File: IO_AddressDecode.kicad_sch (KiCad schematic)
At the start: 42 parts, among them J0 Cassette Data In, J13 74LS74, J14 GAME_IO_Conn, J2 Cassette Data Out, K13 MA741, Q4 MPSA13

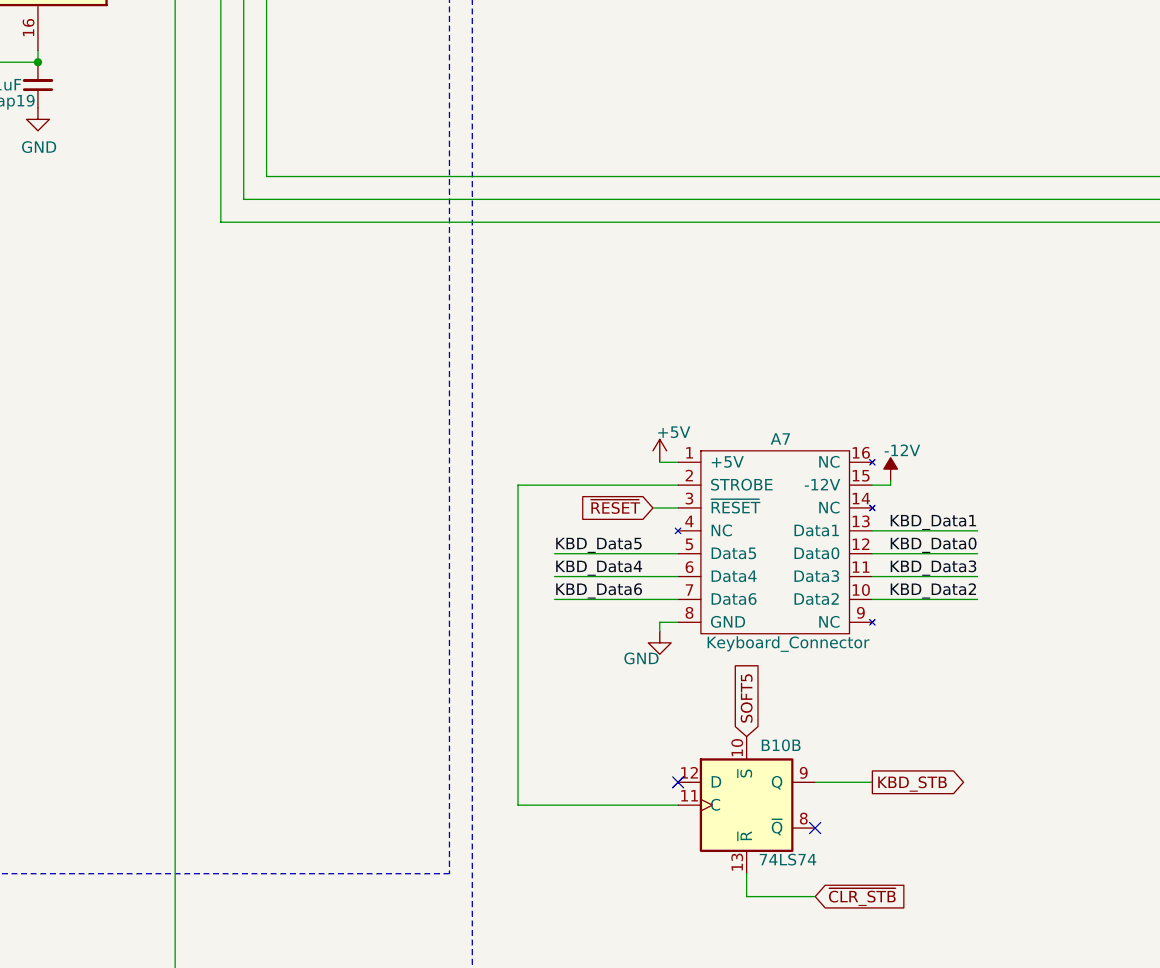
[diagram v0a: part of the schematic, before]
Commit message: finish tracing
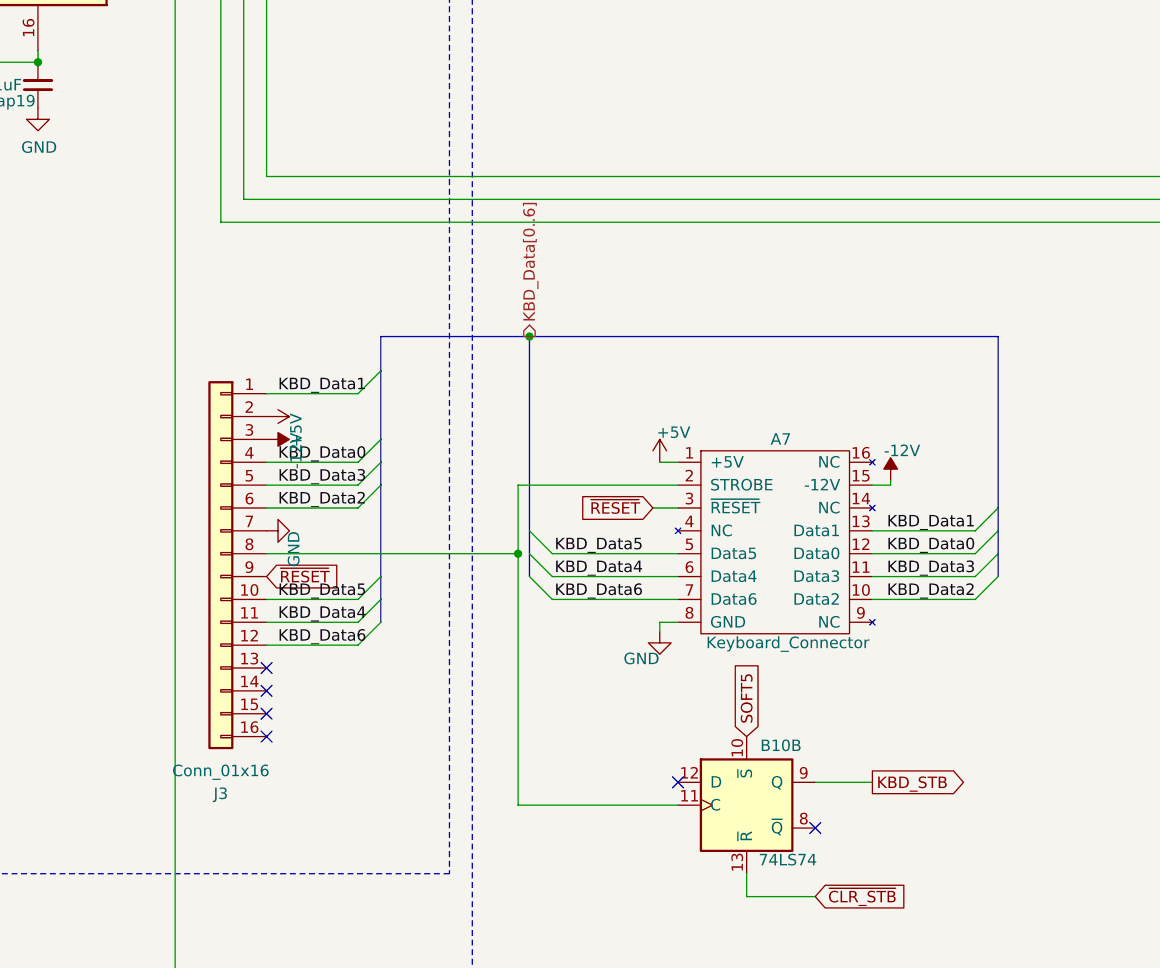
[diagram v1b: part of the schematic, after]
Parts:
- added J3: Conn_01x16, Connector_PinHeader_2.54mm:PinHeader_1x16_P2.54mm_Vertical, symbol Connector_Generic:Conn_01x16
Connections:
- net +5V: now also J3.2 (Pin_2)
- net -12V: now also J3.3 (Pin_3)
- net GND: now also J3.7 (Pin_7)
- net KBD_Data0: now also J3.4 (Pin_4)
- net KBD_Data1: now also J3.1 (Pin_1)
- net KBD_Data2: now also J3.6 (Pin_6)
- net KBD_Data3: now also J3.5 (Pin_5)
- net KBD_Data4: now also J3.11 (Pin_11)
- net KBD_Data5: now also J3.10 (Pin_10)
- net KBD_Data6: now also J3.12 (Pin_12)
- net ~{RESET}: now also J3.9 (Pin_9)
- net at A7.2 (STROBE), B10.11 (C): now also J3.8 (Pin_8)
- no-connect marks 7 -> 11

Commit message: beautify resistors
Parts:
- Cap10, Cap11, Cap12, Cap16, Cap18, Cap19, Cap5, Cap6, Cap7, Cap9: footprint Capacitor_THT:C_Disc_D5.0mm_W2.5mm_P5.00mm -> Apple-II:C_Disc_D5.0mm_W2.5mm_P5.00mm
- Cap8: footprint Capacitor_THT:C_Disc_D4.3mm_W1.9mm_P5.00mm -> Apple-II:C_Disc_D5.0mm_W2.5mm_P5.00mm
- R15, R16, R17, R18, R19, R20, R21, R22, R23, R24, R25, R29: footprint Resistor_THT:R_Axial_DIN0207_L6.3mm_D2.5mm_P10.16mm_Horizontal -> Apple-II:R_Axial_DIN0207_L6.3mm_D2.5mm_P10.16mm_Horizontal
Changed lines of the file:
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@@
       (effects (font (size 1.27 1.27)) (justify left))
     )
-    (property "Footprint" "Capacitor_THT:C_Disc_D5.0mm_W2.5mm_P5.00mm" (at 340.36 167.64 0)
+    (property "Footprint" "Apple-II:C_Disc_D5.0mm_W2.5mm_P5.00mm" (at 340.36 167.64 0)
       (effects (font (size 1.27 1.27)) hide)
     )
@@
       (effects (font (size 1.27 1.27)))
     )
-    (property "Footprint" "Resistor_THT:R_Axial_DIN0207_L6.3mm_D2.5mm_P10.16mm_Horizontal" (at 356.108 100.33 0)
+    (property "Footprint" "Apple-II:R_Axial_DIN0207_L6.3mm_D2.5mm_P10.16mm_Horizontal" (at 356.108 100.33 0)
       (effects (font (size 1.27 1.27)) hide)
     )
@@
       (effects (font (size 1.27 1.27)))
     )
-    (property "Footprint" "Resistor_THT:R_Axial_DIN0207_L6.3mm_D2.5mm_P10.16mm_Horizontal" (at 380.746 94.996 0)
+    (property "Footprint" "Apple-II:R_Axial_DIN0207_L6.3mm_D2.5mm_P10.16mm_Horizontal" (at 380.746 94.996 0)
       (effects (font (size 1.27 1.27)) hide)
     )
@@
       (effects (font (size 1.27 1.27)))
     )
-    (property "Footprint" "Resistor_THT:R_Axial_DIN0207_L6.3mm_D2.5mm_P10.16mm_Horizontal" (at 371.856 84.836 0)
+    (property "Footprint" "Apple-II:R_Axial_DIN0207_L6.3mm_D2.5mm_P10.16mm_Horizontal" (at 371.856 84.836 0)
       (effects (font (size 1.27 1.27)) hide)
     )
@@
       (effects (font (size 1.27 1.27)))
     )
-    (property "Footprint" "Resistor_THT:R_Axial_DIN0207_L6.3mm_D2.5mm_P10.16mm_Horizontal" (at 356.616 78.232 0)
+    (property "Footprint" "Apple-II:R_Axial_DIN0207_L6.3mm_D2.5mm_P10.16mm_Horizontal" (at 356.616 78.232 0)
       (effects (font (size 1.27 1.27)) hide)
     )
@@
       (effects (font (size 1.27 1.27)))
     )
-    (property "Footprint" "Resistor_THT:R_Axial_DIN0207_L6.3mm_D2.5mm_P10.16mm_Horizontal" (at 347.98 167.64 0)
+    (property "Footprint" "Apple-II:R_Axial_DIN0207_L6.3mm_D2.5mm_P10.16mm_Horizontal" (at 347.98 167.64 0)
       (effects (font (size 1.27 1.27)) hide)
     )
@@
       (effects (font (size 1.27 1.27)))
     )
-    (property "Footprint" "Resistor_THT:R_Axial_DIN0207_L6.3mm_D2.5mm_P10.16mm_Horizontal" (at 374.396 162.56 0)
+    (property "Footprint" "Apple-II:R_Axial_DIN0207_L6.3mm_D2.5mm_P10.16mm_Horizontal" (at 374.396 162.56 0)
       (effects (font (size 1.27 1.27)) hide)
     )
@@
       (effects (font (size 1.27 1.27)) (justify left))
     )
-    (property "Footprint" "Capacitor_THT:C_Disc_D5.0mm_W2.5mm_P5.00mm" (at 381 168.91 0)
+    (property "Footprint" "Apple-II:C_Disc_D5.0mm_W2.5mm_P5.00mm" (at 381 168.91 0)
       (effects (font (size 1.27 1.27)) hide)
     )
@@
       (effects (font (size 1.27 1.27)) (justify left))
     )
-    (property "Footprint" "Capacitor_THT:C_Disc_D5.0mm_W2.5mm_P5.00mm" (at 351.282 102.87 0)
+    (property "Footprint" "Apple-II:C_Disc_D5.0mm_W2.5mm_P5.00mm" (at 351.282 102.87 0)
       (effects (font (size 1.27 1.27)) hide)
     )
@@
       (effects (font (size 1.27 1.27)) (justify left))
     )
-    (property "Footprint" "Capacitor_THT:C_Disc_D5.0mm_W2.5mm_P5.00mm" (at 375.412 101.346 0)
+    (property "Footprint" "Apple-II:C_Disc_D5.0mm_W2.5mm_P5.00mm" (at 375.412 101.346 0)
       (effects (font (size 1.27 1.27)) hide)
     )
@@
       (effects (font (size 1.27 1.27)) (justify left))
     )
-    (property "Footprint" "Capacitor_THT:C_Disc_D4.3mm_W1.9mm_P5.00mm" (at 350.012 80.772 0)
+    (property "Footprint" "Apple-II:C_Disc_D5.0mm_W2.5mm_P5.00mm" (at 350.012 80.772 0)
       (effects (font (size 1.27 1.27)) hide)
     )
@@
       (effects (font (size 1.27 1.27)) (justify left))
     )
-    (property "Footprint" "Capacitor_THT:C_Disc_D5.0mm_W2.5mm_P5.00mm" (at 362.204 87.376 0)
+    (property "Footprint" "Apple-II:C_Disc_D5.0mm_W2.5mm_P5.00mm" (at 362.204 87.376 0)
       (effects (font (size 1.27 1.27)) hide)
     )
@@
       (effects (font (size 1.27 1.27)) (justify left))
     )
-    (property "Footprint" "Capacitor_THT:C_Disc_D5.0mm_W2.5mm_P5.00mm" (at 345.186 111.252 0)
+    (property "Footprint" "Apple-II:C_Disc_D5.0mm_W2.5mm_P5.00mm" (at 345.186 111.252 0)
       (effects (font (size 1.27 1.27)) hide)
     )
@@
       (effects (font (size 1.27 1.27)))
     )
-    (property "Footprint" "Resistor_THT:R_Axial_DIN0207_L6.3mm_D2.5mm_P10.16mm_Horizontal" (at 345.44 200.914 0)
+    (property "Footprint" "Apple-II:R_Axial_DIN0207_L6.3mm_D2.5mm_P10.16mm_Horizontal" (at 345.44 200.914 0)
       (effects (font (size 1.27 1.27)) hide)
     )
@@
       (effects (font (size 1.27 1.27)))
     )
-    (property "Footprint" "Resistor_THT:R_Axial_DIN0207_L6.3mm_D2.5mm_P10.16mm_Horizontal" (at 353.06 204.724 0)
+    (property "Footprint" "Apple-II:R_Axial_DIN0207_L6.3mm_D2.5mm_P10.16mm_Horizontal" (at 353.06 204.724 0)
       (effects (font (size 1.27 1.27)) hide)
     )
@@
       (effects (font (size 1.27 1.27)) (justify left))
     )
-    (property "Footprint" "Capacitor_THT:C_Disc_D5.0mm_W2.5mm_P5.00mm" (at 347.98 236.22 0)
+    (property "Footprint" "Apple-II:C_Disc_D5.0mm_W2.5mm_P5.00mm" (at 347.98 236.22 0)
       (effects (font (size 1.27 1.27)) hide)
     )
@@
       (effects (font (size 0.9906 0.9906)))
     )
-    (property "Footprint" "Resistor_THT:R_Axial_DIN0207_L6.3mm_D2.5mm_P10.16mm_Horizontal" (at 328.93 241.3 0)
+    (property "Footprint" "Apple-II:R_Axial_DIN0207_L6.3mm_D2.5mm_P10.16mm_Horizontal" (at 328.93 241.3 0)
       (effects (font (size 1.27 1.27)) hide)
     )
@@
       (effects (font (size 0.9906 0.9906)))
     )
-    (property "Footprint" "Resistor_THT:R_Axial_DIN0207_L6.3mm_D2.5mm_P10.16mm_Horizontal" (at 314.96 223.52 0)
+    (property "Footprint" "Apple-II:R_Axial_DIN0207_L6.3mm_D2.5mm_P10.16mm_Horizontal" (at 314.96 223.52 0)
       (effects (font (size 1.27 1.27)) hide)
     )
@@
       (effects (font (size 0.9906 0.9906)))
     )
-    (property "Footprint" "Resistor_THT:R_Axial_DIN0207_L6.3mm_D2.5mm_P10.16mm_Horizontal" (at 297.18 233.68 0)
+    (property "Footprint" "Apple-II:R_Axial_DIN0207_L6.3mm_D2.5mm_P10.16mm_Horizontal" (at 297.18 233.68 0)
       (effects (font (size 1.27 1.27)) hide)
     )
@@
       (effects (font (size 0.9906 0.9906)))
     )
-    (property "Footprint" "Resistor_THT:R_Axial_DIN0207_L6.3mm_D2.5mm_P10.16mm_Horizontal" (at 334.01 231.14 0)
+    (property "Footprint" "Apple-II:R_Axial_DIN0207_L6.3mm_D2.5mm_P10.16mm_Horizontal" (at 334.01 231.14 0)
       (effects (font (size 1.27 1.27)) hide)
     )
@@
       (effects (font (size 1.27 1.27)) (justify left))
     )
-    (property "Footprint" "Capacitor_THT:C_Disc_D5.0mm_W2.5mm_P5.00mm" (at 325.12 21.59 0)
+    (property "Footprint" "Apple-II:C_Disc_D5.0mm_W2.5mm_P5.00mm" (at 325.12 21.59 0)
       (effects (font (size 1.27 1.27)) hide)
     )
@@
       (effects (font (size 1.27 1.27)) (justify left))
     )
-    (property "Footprint" "Capacitor_THT:C_Disc_D5.0mm_W2.5mm_P5.00mm" (at 168.91 120.65 0)
+    (property "Footprint" "Apple-II:C_Disc_D5.0mm_W2.5mm_P5.00mm" (at 168.91 120.65 0)
       (effects (font (size 1.27 1.27)) hide)
     )
@@
       (effects (font (size 1.27 1.27)) (justify left))
     )
-    (property "Footprint" "Capacitor_THT:C_Disc_D5.0mm_W2.5mm_P5.00mm" (at 57.15 162.56 0)
-      (effects (font (size 1.27 1.27)) hide)
-    )
+    (property "Footprint" "Apple-II:C_Disc_D5.0mm_W2.5mm_P5.00mm" (at 57.15 162.56 0)
+      (effects (font (size 1.27 1.27)) hide)
+    )
